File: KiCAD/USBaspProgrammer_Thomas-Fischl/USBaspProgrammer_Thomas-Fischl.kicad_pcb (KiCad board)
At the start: 2 copper layers, 79.4 x 41.9 mm, 22 parts, among them J1 USB_B, J2 ISP_header_Conn_02x05_Odd_Even, U1 ATmega88-20PU, Y1 12MHz

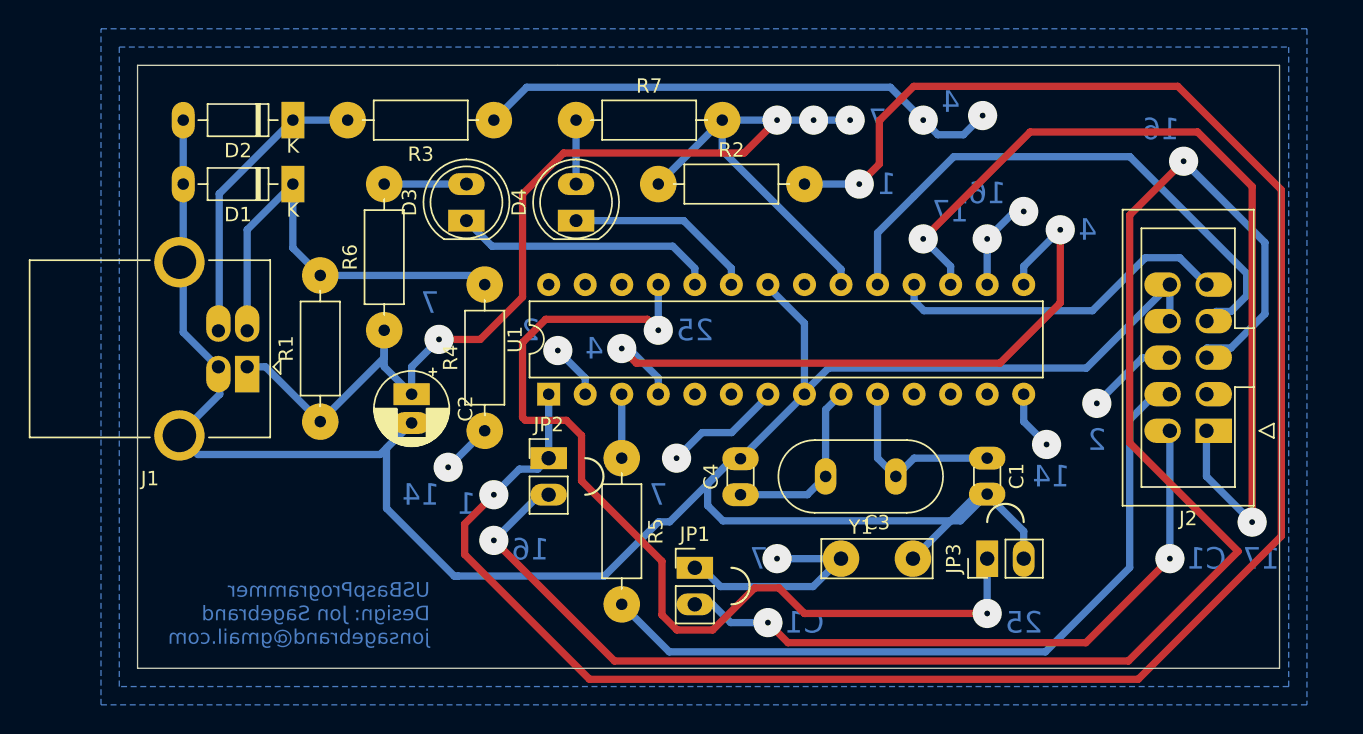
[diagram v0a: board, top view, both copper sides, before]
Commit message: devBoard, gerbers
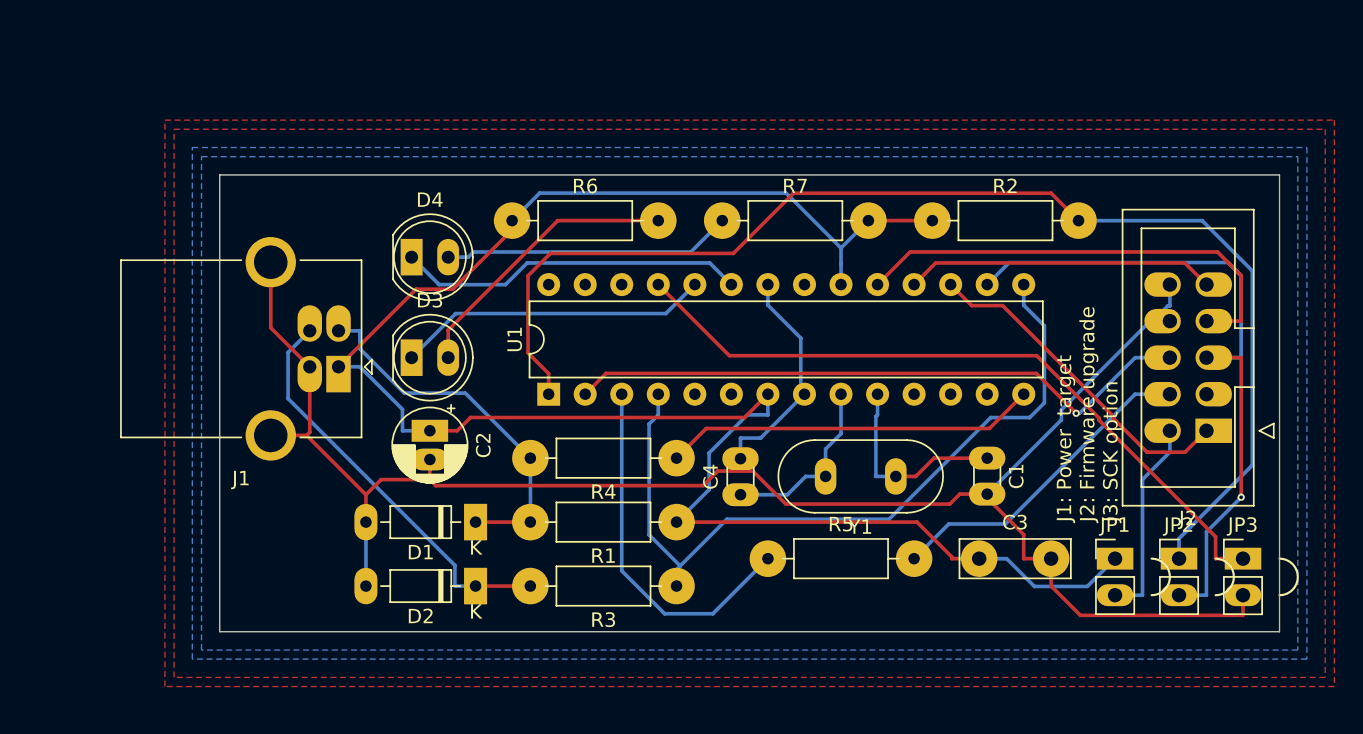
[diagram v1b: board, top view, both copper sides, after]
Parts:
- moved JP2 44.4 mm to (181.6, 123.8)
- moved D2 34.8 mm to (132.7, 125.7)
- moved R3 34.8 mm to (146.7, 125.7)
- moved JP1 29.2 mm to (177.2, 123.8)
- moved D1 26.7 mm to (132.7, 121.3)
- moved R1 25.7 mm to (146.7, 121.3), turned to 180 degrees
- moved R2 19.2 mm to (164.5, 100.3)
- moved JP3 17.8 mm to (186.1, 123.8), turned to 0 degrees
- moved R4 13.5 mm to (146.7, 116.8), turned to 180 degrees
- moved R7 12.3 mm to (149.9, 100.3)
- moved R5 12.3 mm to (153.0, 123.8), turned to 0 degrees
- moved R6 11.7 mm to (135.3, 100.3), turned to 0 degrees
- moved D4 11.7 mm to (128.3, 102.9), turned to 0 degrees
- moved D3 10.3 mm to (128.3, 109.9), turned to 0 degrees
- moved C3 9.60 mm to (167.7, 123.8)
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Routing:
- net Net-(J2-Pad5): track 120.9 -> 48.6 mm, vias 4 -> 1
- net Net-(JP2-Pad1): track 143.6 -> 85.9 mm, vias 2 -> 0
- net Net-(J2-Pad1): track 62.5 -> 23.3 mm, vias 2 -> 0
- net Net-(J2-Pad6): track 10.2 -> 44.0 mm, vias 2 -> 1
- net Net-(R3-Pad1): track 85.3 -> 53.4 mm, vias 4 -> 0
- net Net-(J2-Pad2): track 45.4 -> 14.1 mm, vias 2 -> 0
- net Net-(J2-Pad4): track 52.9 -> 22.5 mm
- net GND: track 161.8 -> 137.7 mm
- net Net-(R5-Pad1): track 4.45 -> 25.3 mm
- net +5V: track 112.9 -> 130.7 mm, vias 6 -> 0
- net Net-(R4-Pad1): track 8.19 -> 26.0 mm, vias 2 -> 0
- net Net-(JP3-Pad1): track 67.0 -> 49.5 mm, vias 2 -> 0
- net Net-(D4-Pad2): track 4.45 -> 20.1 mm
- net Net-(D3-Pad2): track 5.72 -> 19.7 mm
- net RedLED: track 13.3 -> 24.3 mm
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- added copper zone on F.Cu, net (none)
- added copper zone on F.Cu, net GND
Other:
- board size 79.4 x 41.9 mm -> 73.7 x 31.8 mm
- net class Default: clearance 0.762 -> 0.508; trace_width 0.508 -> 0.254; via_dia 2.032 -> 0.508
- rule trace_clearance: 0.762 -> 0.508
- board text added: "J1: Power target J2: Firmware upgrade J3: SCK option"
- board text removed: "1"
- board text removed: "14"
- board text removed: "16"
- board text removed: "17"
- board text removed: "2"
- board text removed: "25"
- board text removed: "4"
- board text removed: "7"
- board text removed: "C1"
